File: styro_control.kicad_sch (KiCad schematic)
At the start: 89 parts, among them J3 INPUT_PEDAL, Q1 IRF7324, SW1 SW_RESET, SW2 switch_6_pin, SW3 SW_1, SW4 SW_2, SW5 SW_3, U1 STUSB4500QTR, U2 PAC1932-4, U3 ATSAMD21E18A-M, U4 INA226, Y1 Crystal

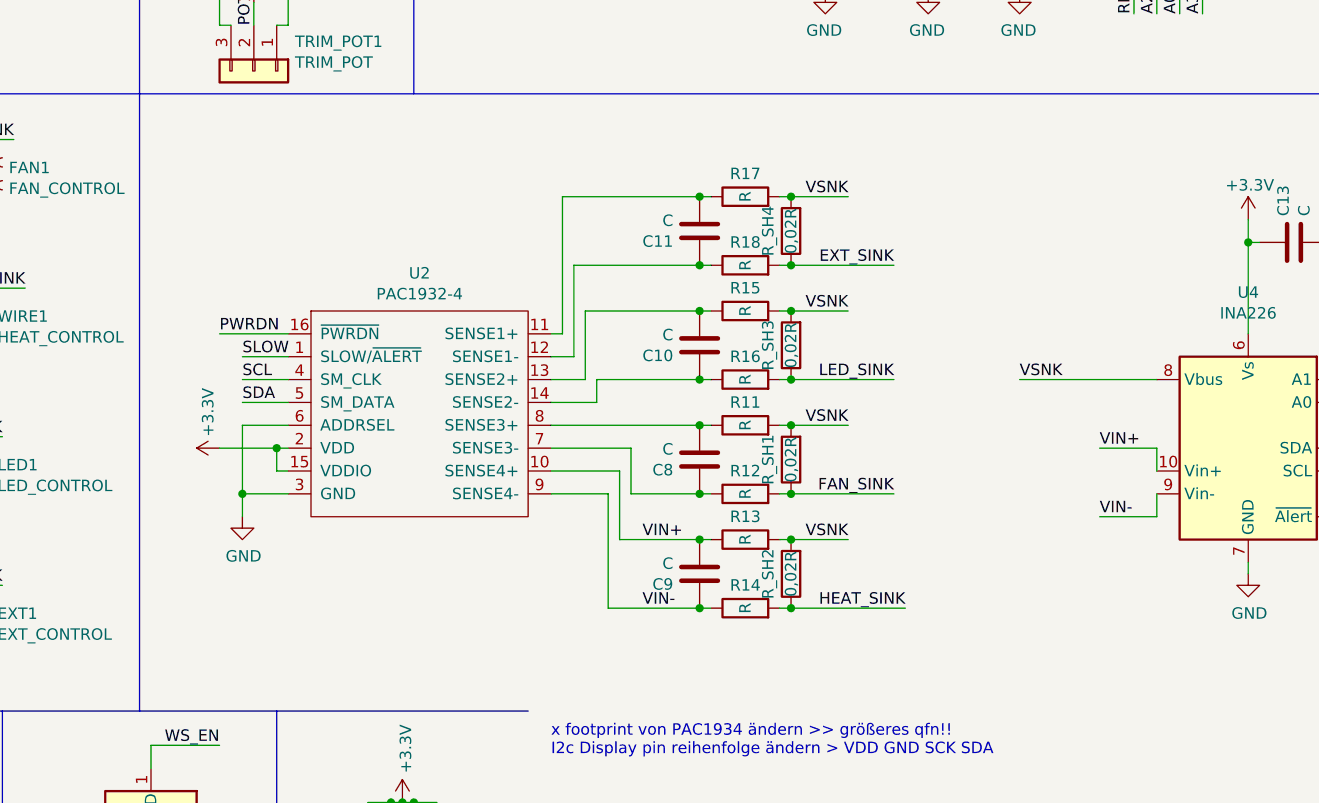
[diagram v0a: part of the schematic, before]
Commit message: updated schematic
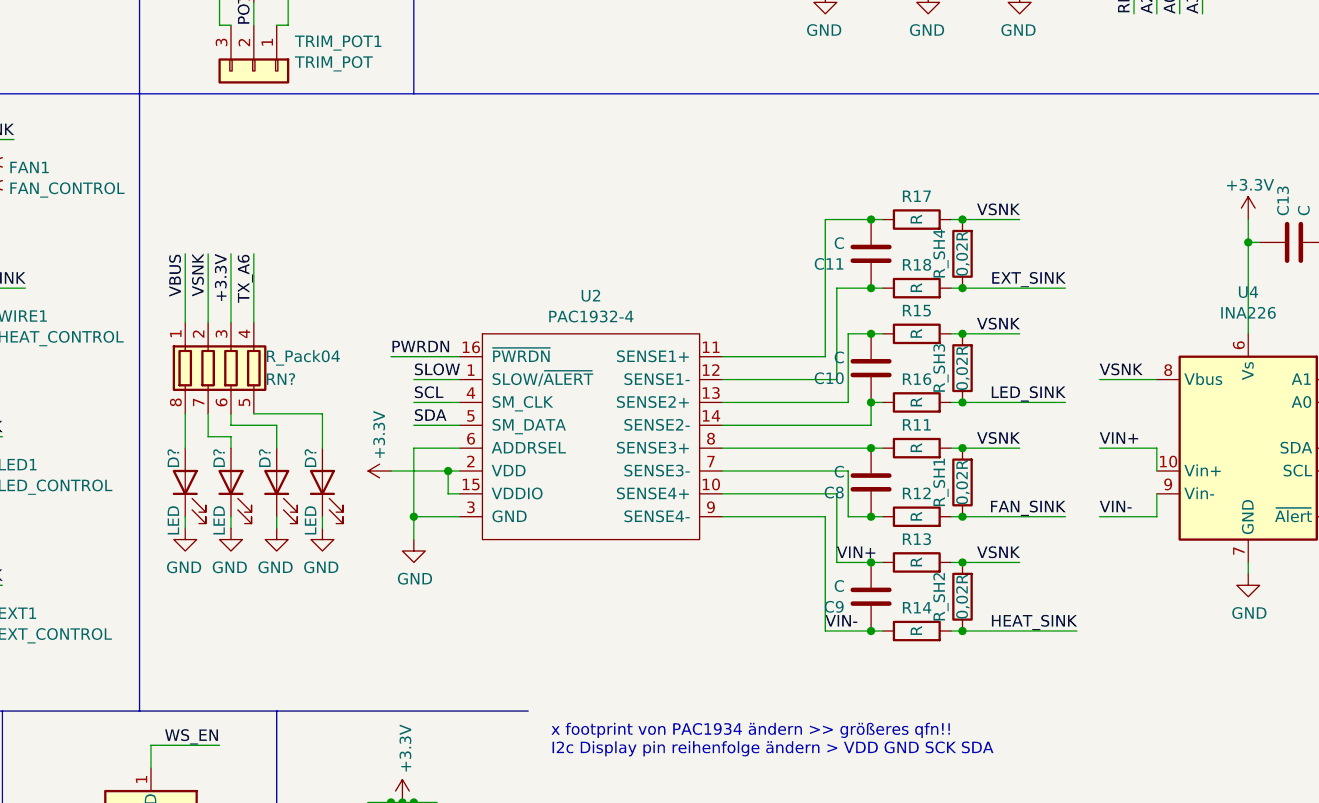
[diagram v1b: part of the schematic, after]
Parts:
- added D? (x3): LED, symbol Device:LED
- added D?: (no value), symbol Device:LED
- added RN?: R_Pack04, Resistor_SMD:R_Array_Convex_4x0603, symbol Device:R_Pack04
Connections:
- net GND: now also D?.1 (K), D?.1 (K), D?.1 (K), D?.1 (K)
- net TX_A6: now also RN?.4 (R4.1)
- net VBUS: now also RN?.1 (R1.1)
- net VSNK: now also RN?.2 (R2.1)
- new net: D?.2 (A), RN?.8 (R1.2)
- new net: D?.2 (A), RN?.7 (R2.2)
- new net: D?.2 (A), RN?.6 (R3.2)
- new net: D?.2 (A), RN?.5 (R4.2)
- new net +3.3V: RN?.3 (R3.1)
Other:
- moved on the sheet: C10, C11, C8, C9, R11, R12, R13, R14, R15, R16, R17, R18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
